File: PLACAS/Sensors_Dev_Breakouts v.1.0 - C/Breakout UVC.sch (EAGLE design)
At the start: 5 parts

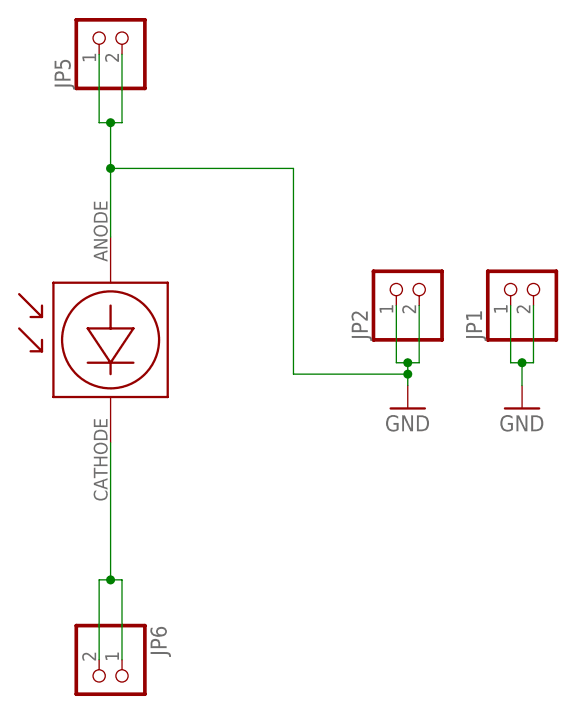
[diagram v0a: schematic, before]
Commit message: Add files via upload
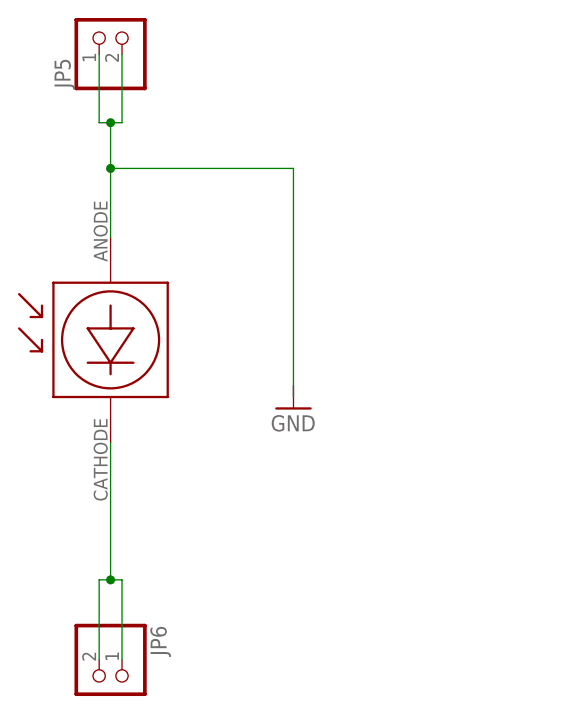
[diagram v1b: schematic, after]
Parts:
- removed JP1, JP2: (no value), pinhead(1x3):PINHD-1X2
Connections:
- net GND: no longer JP1.1, JP1.2, JP2.1, JP2.2
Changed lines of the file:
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@@
 <parts>
 <part name="U$1" library="GUVX" deviceset="GUVC-S10GD" device=""/>
-<part name="JP1" library="pinhead(1x3)" deviceset="PINHD-1X2" device="" package3d_urn="urn:adsk.eagle:package:22435/2"/>
-<part name="JP2" library="pinhead(1x3)" deviceset="PINHD-1X2" device="" package3d_urn="urn:adsk.eagle:package:22435/2"/>
-<part name="GND1" library="supply1" library_urn="urn:adsk.eagle:library:371" deviceset="GND" device=""/>
 <part name="GND2" library="supply1" library_urn="urn:adsk.eagle:library:371" deviceset="GND" device=""/>
 <part name="JP5" library="pinhead(1x3)" deviceset="PINHD-1X2" device="" package3d_urn="urn:adsk.eagle:package:22435/2"/>
@@
 <instances>
 <instance part="U$1" gate="G$1" x="86.36" y="50.8" smashed="yes"/>
-<instance part="JP1" gate="G$1" x="140.97" y="50.8" smashed="yes" rot="R90">
-<attribute name="NAME" x="135.255" y="44.45" size="1.778" layer="95" rot="R90"/>
-<attribute name="VALUE" x="146.05" y="44.45" size="1.778" layer="96" rot="R90"/>
-</instance>
-<instance part="JP2" gate="G$1" x="128.27" y="50.8" smashed="yes" rot="R90">
-<attribute name="NAME" x="122.555" y="44.45" size="1.778" layer="95" rot="R90"/>
-<attribute name="VALUE" x="133.35" y="44.45" size="1.778" layer="96" rot="R90"/>
-</instance>
-<instance part="GND1" gate="1" x="127" y="36.83" smashed="yes">
-<attribute name="VALUE" x="124.46" y="34.29" size="1.778" layer="96"/>
-</instance>
-<instance part="GND2" gate="1" x="139.7" y="36.83" smashed="yes">
-<attribute name="VALUE" x="137.16" y="34.29" size="1.778" layer="96"/>
+<instance part="GND2" gate="1" x="114.3" y="36.83" smashed="yes">
+<attribute name="VALUE" x="111.76" y="34.29" size="1.778" layer="96"/>
 </instance>
 <instance part="JP5" gate="G$1" x="95.25" y="78.74" smashed="yes" rot="R90">
@@
 </busses>
 <nets>
-<net name="GND" class="0">
-<segment>
-<pinref part="JP2" gate="G$1" pin="1"/>
-<wire x1="125.73" y1="48.26" x2="125.73" y2="41.91" width="0.1524" layer="91"/>
-<wire x1="125.73" y1="41.91" x2="127" y2="41.91" width="0.1524" layer="91"/>
-<pinref part="GND1" gate="1" pin="GND"/>
-<wire x1="127" y1="41.91" x2="127" y2="40.64" width="0.1524" layer="91"/>
-<pinref part="JP2" gate="G$1" pin="2"/>
-<wire x1="127" y1="40.64" x2="127" y2="39.37" width="0.1524" layer="91"/>
-<wire x1="127" y1="41.91" x2="128.27" y2="41.91" width="0.1524" layer="91"/>
-<wire x1="128.27" y1="41.91" x2="128.27" y2="48.26" width="0.1524" layer="91"/>
-<junction x="127" y="41.91"/>
-<pinref part="JP5" gate="G$1" pin="1"/>
-<wire x1="92.71" y1="76.2" x2="92.71" y2="68.58" width="0.1524" layer="91"/>
-<pinref part="JP5" gate="G$1" pin="2"/>
-<wire x1="92.71" y1="68.58" x2="93.98" y2="68.58" width="0.1524" layer="91"/>
-<wire x1="93.98" y1="68.58" x2="95.25" y2="68.58" width="0.1524" layer="91"/>
-<wire x1="95.25" y1="68.58" x2="95.25" y2="76.2" width="0.1524" layer="91"/>
-<pinref part="U$1" gate="G$1" pin="ANODE"/>
-<wire x1="93.98" y1="55.88" x2="93.98" y2="63.5" width="0.1524" layer="91"/>
-<junction x="93.98" y="68.58"/>
-<wire x1="93.98" y1="63.5" x2="93.98" y2="68.58" width="0.1524" layer="91"/>
-<wire x1="93.98" y1="63.5" x2="114.3" y2="63.5" width="0.1524" layer="91"/>
-<wire x1="114.3" y1="63.5" x2="114.3" y2="40.64" width="0.1524" layer="91"/>
-<junction x="93.98" y="63.5"/>
-<wire x1="114.3" y1="40.64" x2="127" y2="40.64" width="0.1524" layer="91"/>
-<junction x="127" y="40.64"/>
-</segment>
-<segment>
-<pinref part="JP1" gate="G$1" pin="1"/>
-<wire x1="138.43" y1="48.26" x2="138.43" y2="41.91" width="0.1524" layer="91"/>
-<wire x1="138.43" y1="41.91" x2="139.7" y2="41.91" width="0.1524" layer="91"/>
-<pinref part="GND2" gate="1" pin="GND"/>
-<wire x1="139.7" y1="41.91" x2="139.7" y2="39.37" width="0.1524" layer="91"/>
-<pinref part="JP1" gate="G$1" pin="2"/>
-<wire x1="139.7" y1="41.91" x2="140.97" y2="41.91" width="0.1524" layer="91"/>
-<wire x1="140.97" y1="41.91" x2="140.97" y2="48.26" width="0.1524" layer="91"/>
-<junction x="139.7" y="41.91"/>
-</segment>
-</net>
 <net name="N$2" class="0">
 <segment>
@@
 </segment>
 </net>
+<net name="GND" class="0">
+<segment>
+<pinref part="JP5" gate="G$1" pin="1"/>
+<wire x1="92.71" y1="76.2" x2="92.71" y2="68.58" width="0.1524" layer="91"/>
+<pinref part="JP5" gate="G$1" pin="2"/>
+<wire x1="92.71" y1="68.58" x2="93.98" y2="68.58" width="0.1524" layer="91"/>
+<wire x1="93.98" y1="68.58" x2="95.25" y2="68.58" width="0.1524" layer="91"/>
+<wire x1="95.25" y1="68.58" x2="95.25" y2="76.2" width="0.1524" layer="91"/>
+<pinref part="U$1" gate="G$1" pin="ANODE"/>
+<wire x1="93.98" y1="55.88" x2="93.98" y2="63.5" width="0.1524" layer="91"/>
+<junction x="93.98" y="68.58"/>
+<wire x1="93.98" y1="63.5" x2="93.98" y2="68.58" width="0.1524" layer="91"/>
+<wire x1="93.98" y1="63.5" x2="114.3" y2="63.5" width="0.1524" layer="91"/>
+<wire x1="114.3" y1="63.5" x2="114.3" y2="39.37" width="0.1524" layer="91"/>
+<junction x="93.98" y="63.5"/>
+<pinref part="GND2" gate="1" pin="GND"/>
+<wire x1="114.3" y1="39.37" x2="114.3" y2="38.1" width="0.1524" layer="91"/>
+</segment>
+</net>
